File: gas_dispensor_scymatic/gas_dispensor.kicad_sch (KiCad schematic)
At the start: 9 parts, among them J1 Safety 02 sensor 0x74, J2 Main O2 sensor 0x70, J3 Gas solenoid, J4 Sounder and beacon, K1 5v Relay, K2 5v Relay

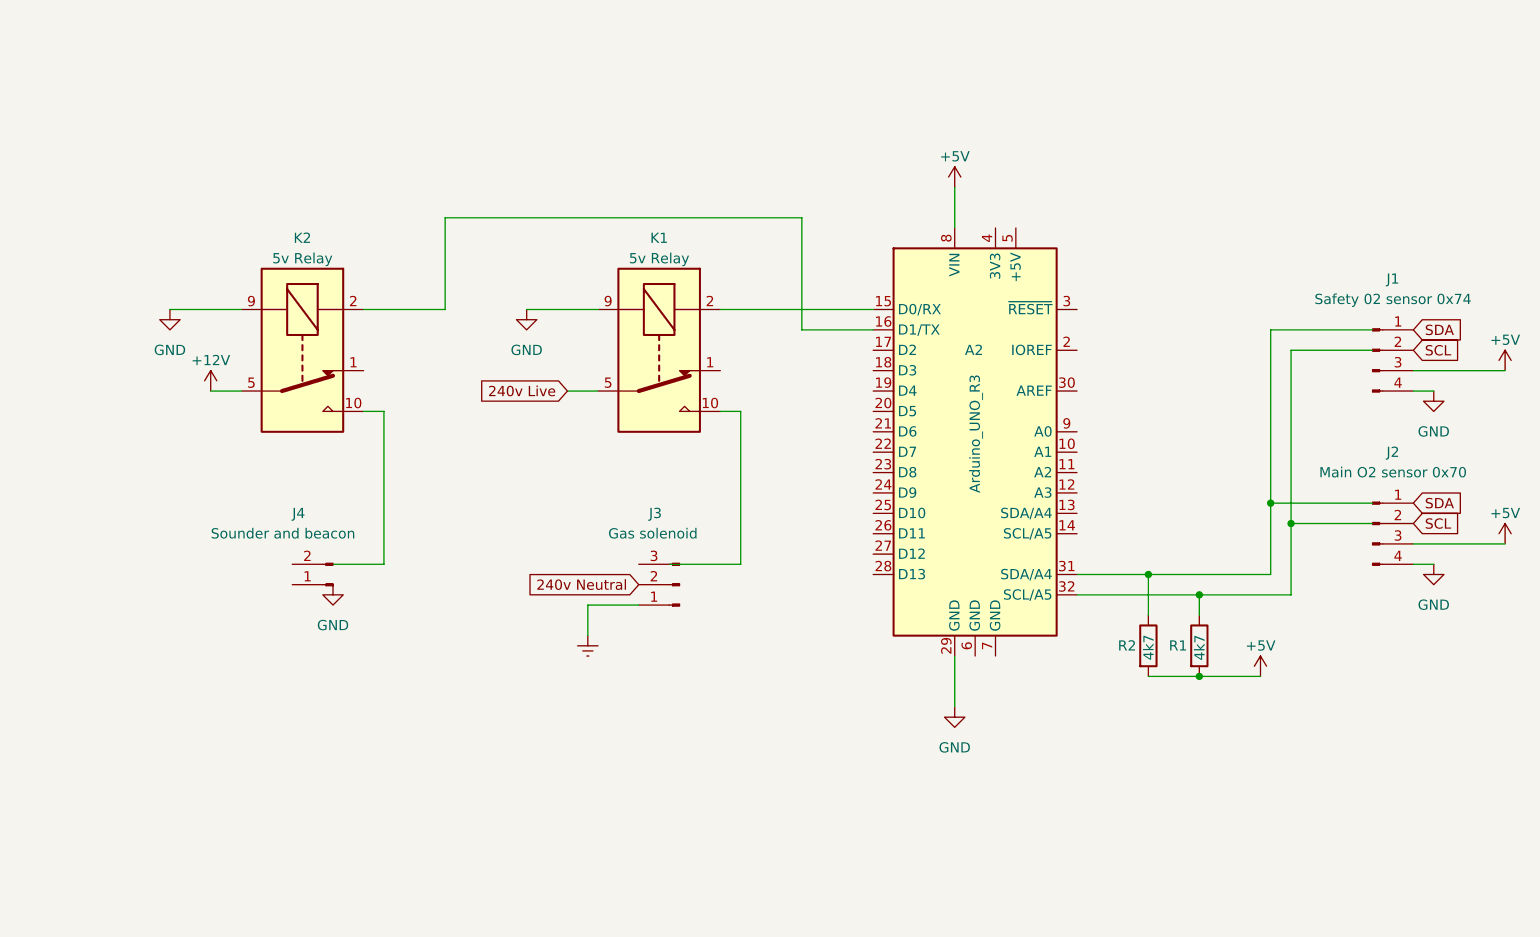
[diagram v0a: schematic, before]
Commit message: added new schymatic
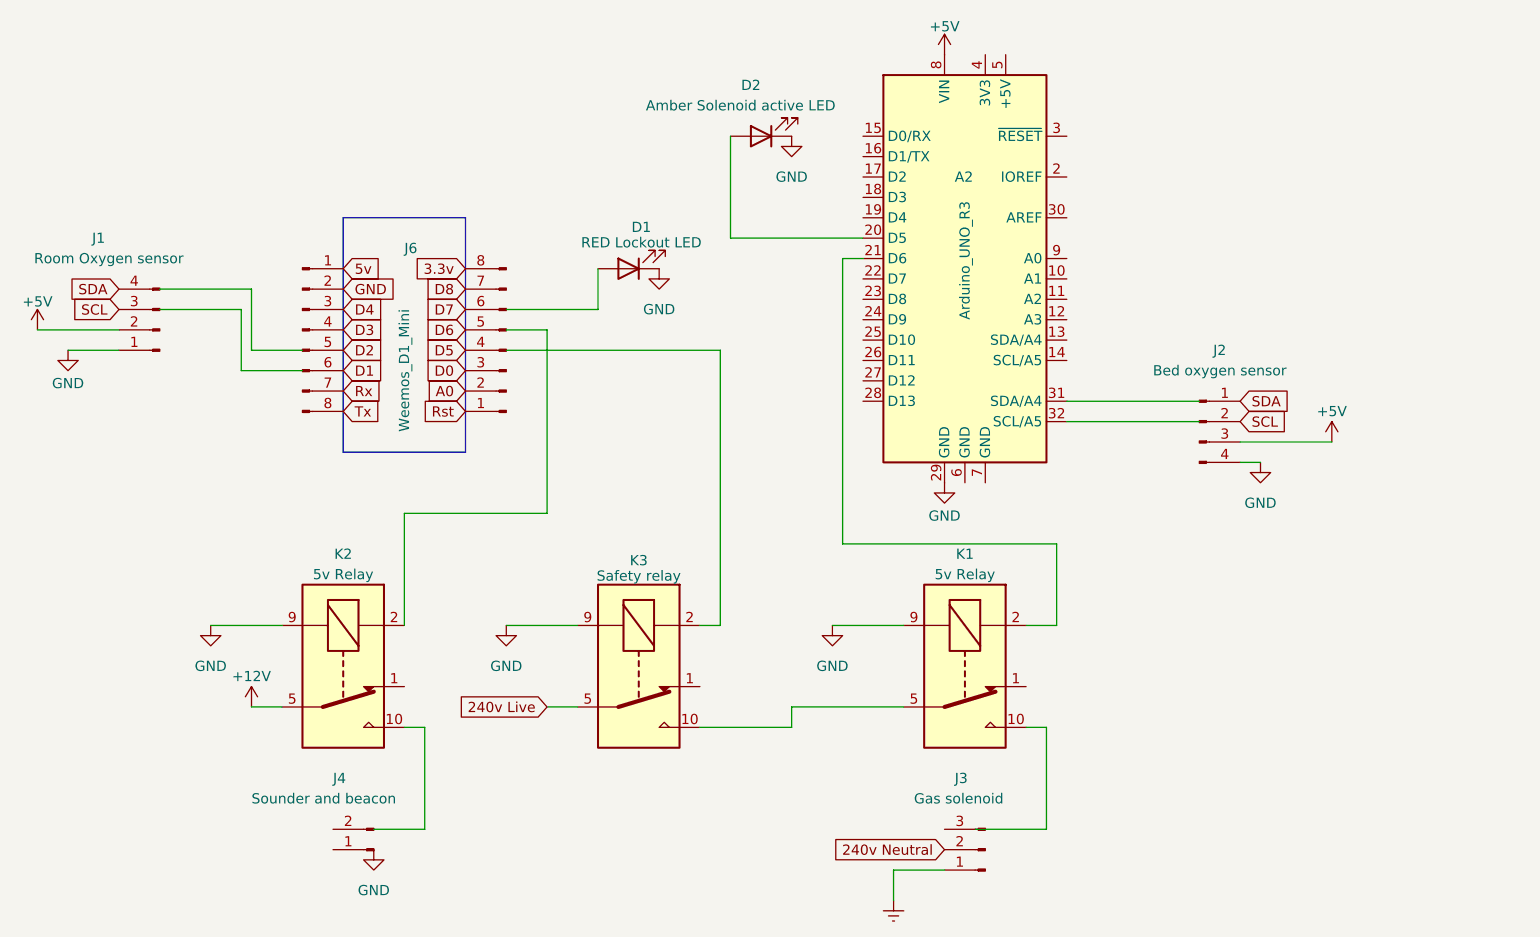
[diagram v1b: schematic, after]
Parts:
- removed R1, R2: 4k7, symbol Device:R
- added D1: RED Lockout LED, symbol Device:LED
- added D2: Amber Solenoid active LED, symbol Device:LED
- added J5: ~, symbol Connector:Conn_01x08_Pin
- added J6: Weemos_D1_Mini, symbol Connector:Conn_01x08_Pin
- added K3: Safety relay, Relay_THT:Relay_SPDT_Omron_G5V-1, symbol Relay:G5V-1
- J1: value Safety 02 sensor 0x74 -> Room Oxygen sensor
- J2: value Main O2 sensor 0x70 -> Bed oxygen sensor
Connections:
- net +5V: now also J1.2 (Pin_2); no longer J1.3 (Pin_3)
- net 240v Live: now also K3.5, K3.6; no longer K1.5, K1.6
- net GND: now also J1.1 (Pin_1), D1.1 (K), D2.1 (K), J5.2 (Pin_2), K3.9; no longer J1.4 (Pin_4)
- net SCL: now also J1.3 (Pin_3); no longer J1.2 (Pin_2)
- net SDA: now also J1.4 (Pin_4); no longer J1.1 (Pin_1)
- net at K1.2: now also A2.21 (D6); no longer A2.15 (D0/RX)
- net at K2.2: no longer A2.16 (D1/TX)
- net at A2.20 (D5): now also D2.2 (A)
- new net: K1.5, K1.6, K3.10
- new net 3.3v: J6.8 (Pin_8)
- new net 5v: J5.1 (Pin_1)
- new net A0: J6.2 (Pin_2)
- new net D0: J6.3 (Pin_3)
- new net D1: J5.6 (Pin_6)
- new net D2: J5.5 (Pin_5)
- new net D3: J5.4 (Pin_4)
- new net D4: J5.3 (Pin_3)
- new net D5: J6.4 (Pin_4)
- new net D6: J6.5 (Pin_5)
- new net D7: J6.6 (Pin_6)
- new net D8: J6.7 (Pin_7)
- new net Rst: J6.1 (Pin_1)
- new net Rx: J5.7 (Pin_7)
- new net Tx: J5.8 (Pin_8)
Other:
- moved on the sheet: A2, J1, J2, J3, J4, K1, K2
